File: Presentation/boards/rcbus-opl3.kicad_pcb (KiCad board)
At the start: 2 copper layers, 100 x 50 mm, 38 parts, among them CON1 3.5mm jack, P1 RC2014 BUS, U1 TL074, U2 YAC512, U3 74HCT688, U4 YMF262, Y1 14.3181MHz

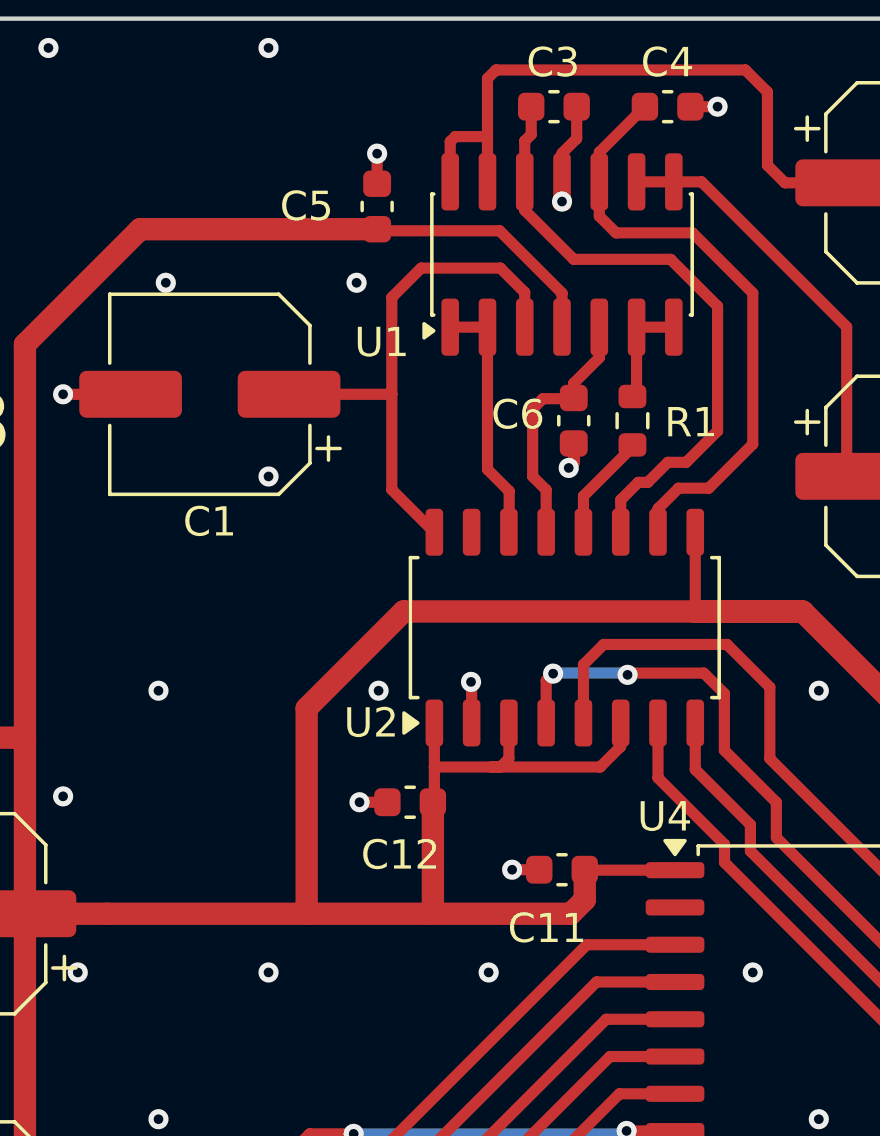
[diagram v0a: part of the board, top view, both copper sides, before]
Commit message: Deploying to main from @ electrified/rcbus-opl3@6dc36e7be147e4cae15e6f13cab98d536f6d43da 🚀
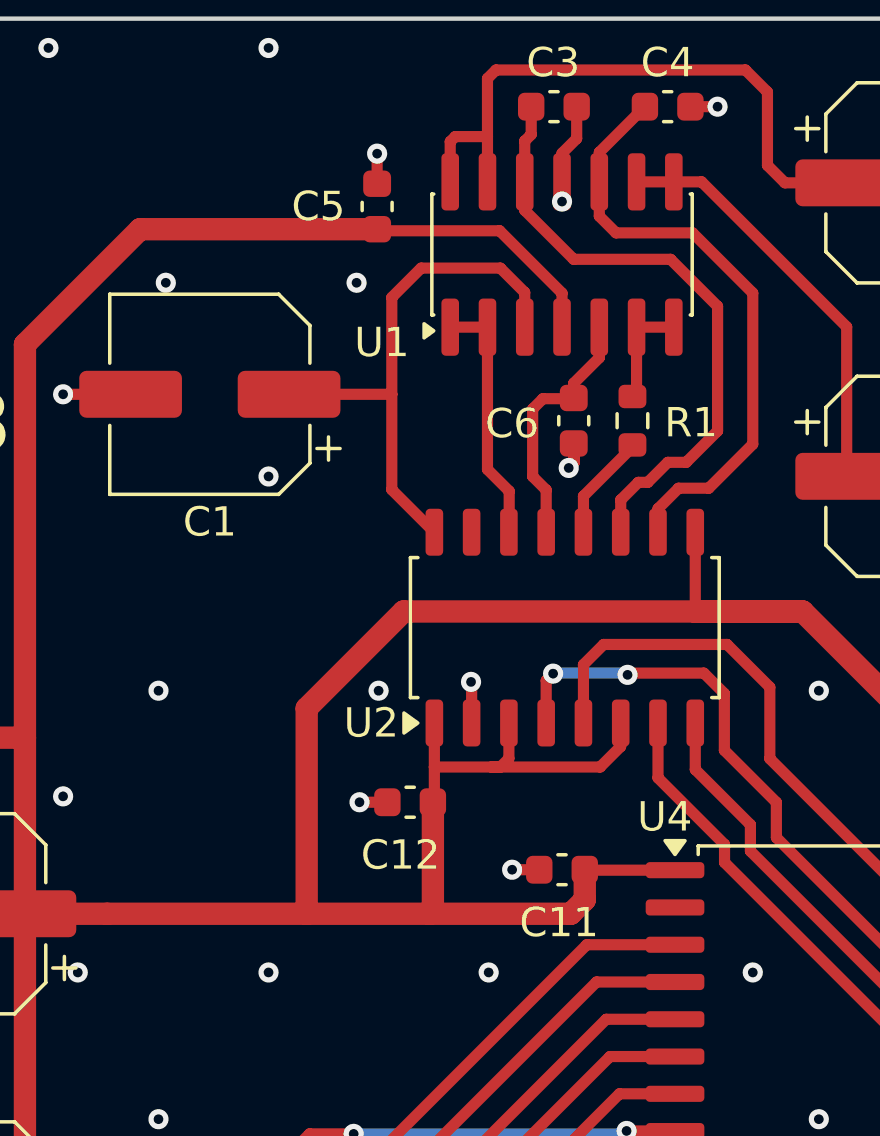
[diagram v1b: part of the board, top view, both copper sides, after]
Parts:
- moved G3 1.00 mm to (104.5, 159.0)
- moved G4 1.00 mm to (98.5, 159.0)
- moved G5 1.00 mm to (92.5, 159.0)
